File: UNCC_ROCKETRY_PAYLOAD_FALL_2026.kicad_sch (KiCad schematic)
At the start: 0 parts

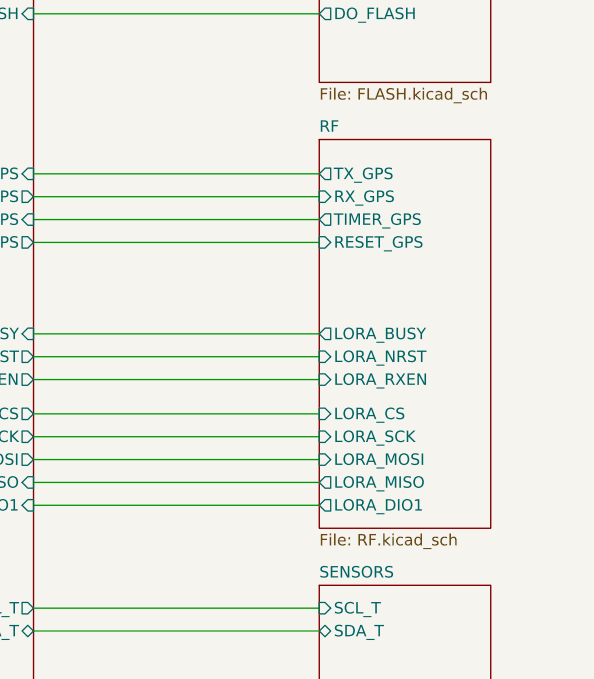
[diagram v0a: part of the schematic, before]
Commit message: started layout
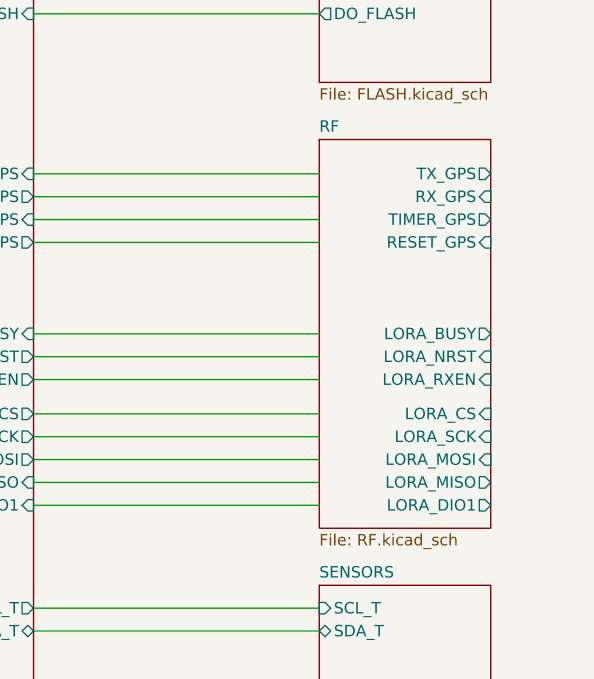
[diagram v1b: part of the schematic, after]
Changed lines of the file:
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@@
 		)
 		(pin "TX_GPS" output
-			(at 190.5 73.66 180)
+			(at 209.55 73.66 0)
 			(effects
 				(font
 					(size 1.27 1.27)
 				)
-				(justify left)
+				(justify right)
 			)
 		)
 		(pin "RX_GPS" input
-			(at 190.5 76.2 180)
+			(at 209.55 76.2 0)
 			(effects
 				(font
 					(size 1.27 1.27)
 				)
-				(justify left)
+				(justify right)
 			)
 		)
 		(pin "TIMER_GPS" output
-			(at 190.5 78.74 180)
+			(at 209.55 78.74 0)
 			(effects
 				(font
 					(size 1.27 1.27)
 				)
-				(justify left)
+				(justify right)
 			)
 		)
 		(pin "RESET_GPS" input
-			(at 190.5 81.28 180)
+			(at 209.55 81.28 0)
 			(effects
 				(font
 					(size 1.27 1.27)
 				)
-				(justify left)
+				(justify right)
 			)
 		)
 		(pin "LORA_RXEN" input
-			(at 190.5 96.52 180)
+			(at 209.55 96.52 0)
 			(effects
 				(font
 					(size 1.27 1.27)
 				)
-				(justify left)
+				(justify right)
 			)
 		)
 		(pin "LORA_CS" input
-			(at 190.5 100.33 180)
+			(at 209.55 100.33 0)
 			(effects
 				(font
 					(size 1.27 1.27)
 				)
-				(justify left)
+				(justify right)
 			)
 		)
 		(pin "LORA_SCK" input
-			(at 190.5 102.87 180)
+			(at 209.55 102.87 0)
 			(effects
 				(font
 					(size 1.27 1.27)
 				)
-				(justify left)
+				(justify right)
 			)
 		)
 		(pin "LORA_MOSI" input
-			(at 190.5 105.41 180)
+			(at 209.55 105.41 0)
 			(effects
 				(font
 					(size 1.27 1.27)
 				)
-				(justify left)
+				(justify right)
 			)
 		)
 		(pin "LORA_MISO" output
-			(at 190.5 107.95 180)
+			(at 209.55 107.95 0)
 			(effects
 				(font
 					(size 1.27 1.27)
 				)
-				(justify left)
+				(justify right)
 			)
 		)
 		(pin "LORA_BUSY" output
-			(at 190.5 91.44 180)
+			(at 209.55 91.44 0)
 			(effects
 				(font
 					(size 1.27 1.27)
 				)
-				(justify left)
+				(justify right)
 			)
 		)
 		(pin "LORA_DIO1" output
-			(at 190.5 110.49 180)
+			(at 209.55 110.49 0)
 			(effects
 				(font
 					(size 1.27 1.27)
 				)
-				(justify left)
+				(justify right)
 			)
 		)
 		(pin "LORA_NRST" input
-			(at 190.5 93.98 180)
+			(at 209.55 93.98 0)
 			(effects
 				(font
 					(size 1.27 1.27)
 				)
-				(justify left)
+				(justify right)
 			)
 		)
